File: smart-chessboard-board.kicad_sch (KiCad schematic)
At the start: 11 parts, among them J101 Conn_01x12_MountingPin, SW101 SW_SPDT, SW102 SW_SPDT, U101 LTR-F216A, U102 74AHCT1G125

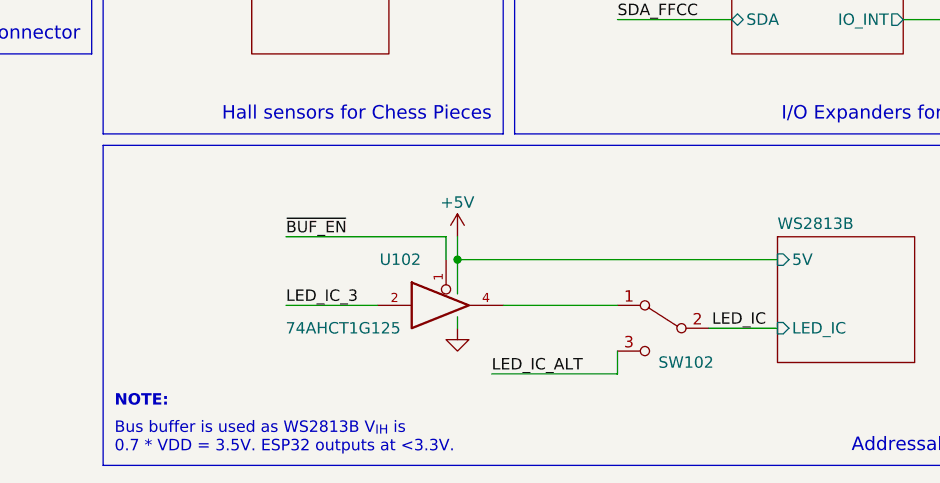
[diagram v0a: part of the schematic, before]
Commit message: update datasheet and parts
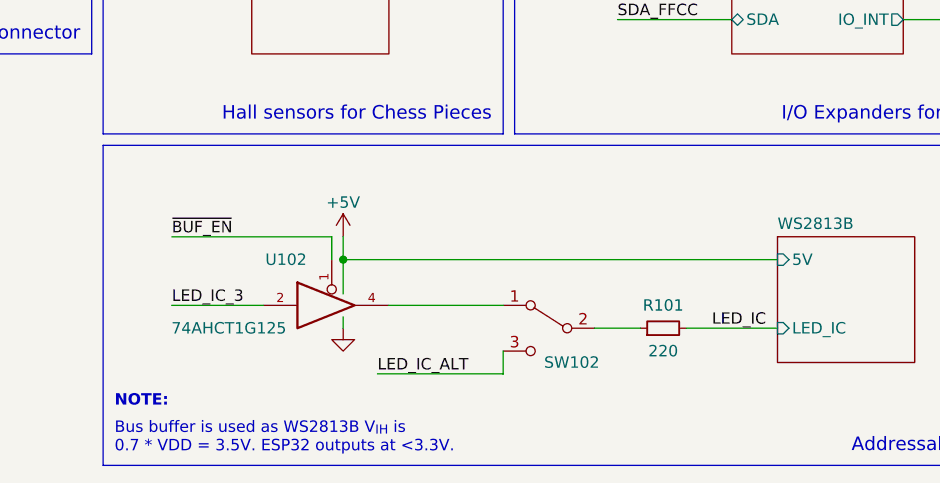
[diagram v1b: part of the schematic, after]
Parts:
- added R101: 220, symbol Device:R_Small
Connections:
- net LED_IC: now also R101.2; no longer SW102.2 (B)
- new net: R101.1, SW102.2 (B)
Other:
- moved on the sheet: SW102, U102
